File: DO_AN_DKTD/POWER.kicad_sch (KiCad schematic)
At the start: 24 parts, among them J2 Jack-DC, J3 Conn_01x07, Q10 P_Mosfet, U1 AMS1117, U1 XL1509

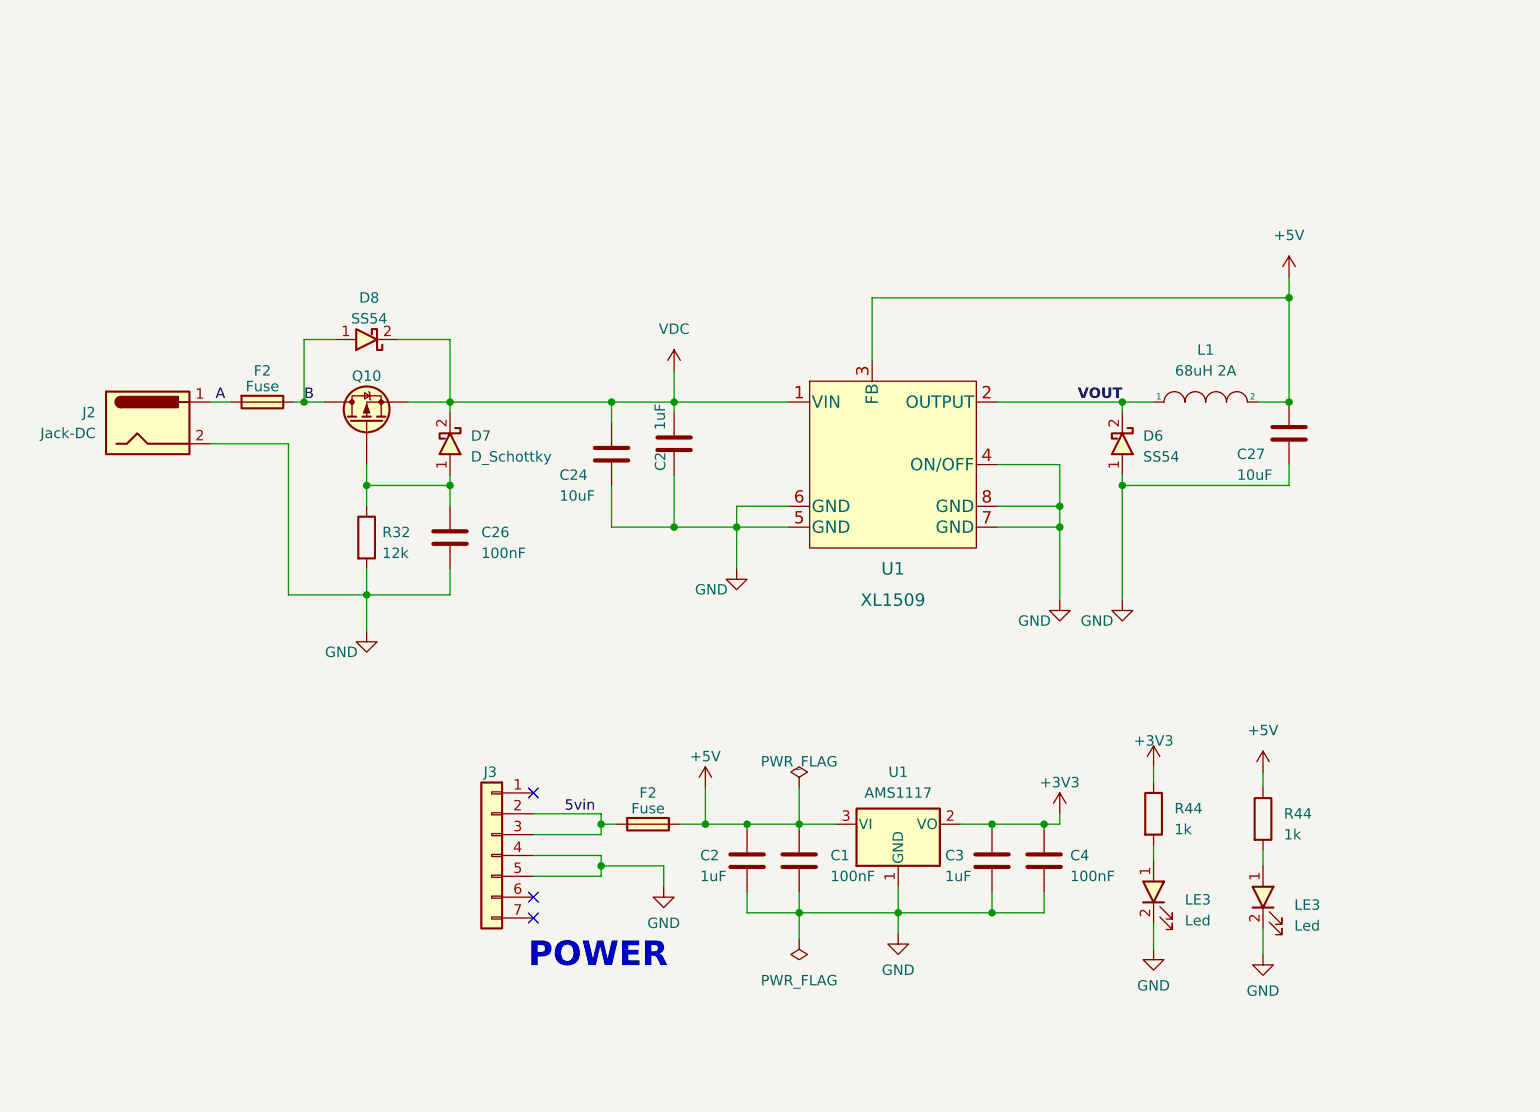
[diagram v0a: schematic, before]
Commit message: commit to change branch
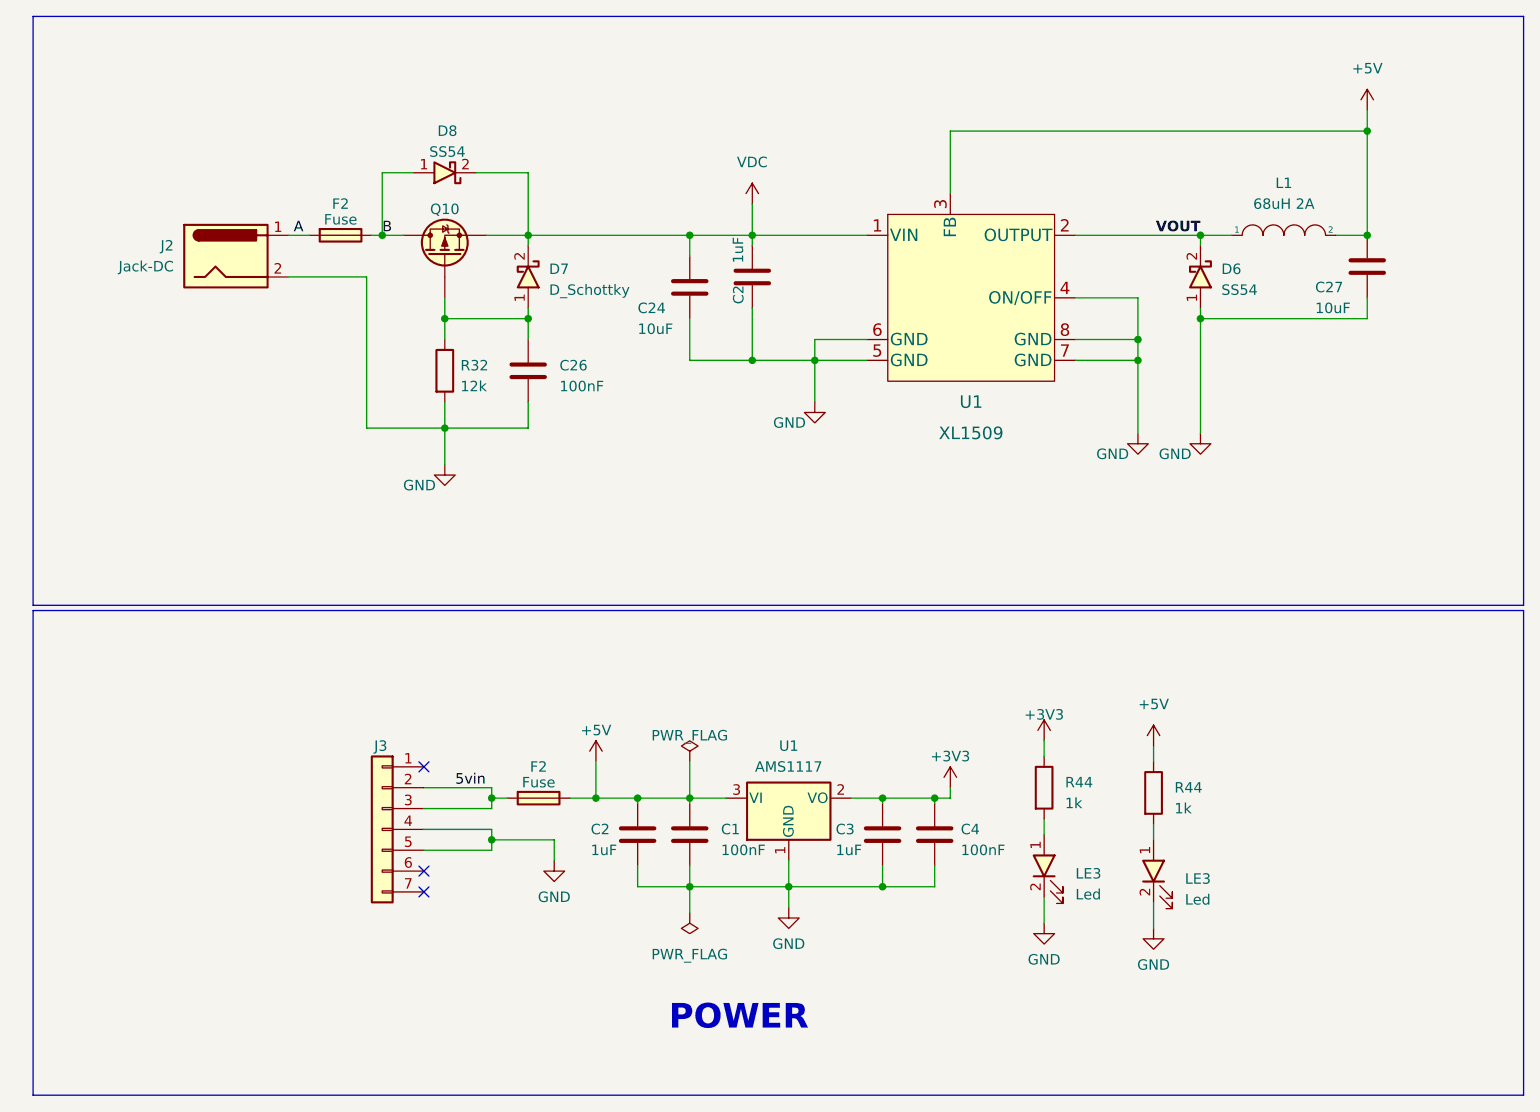
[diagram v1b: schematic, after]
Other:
- moved on the sheet: C1, C2, C24, C26, C27, C3, C4, D6, D7, D8, F2, J2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
